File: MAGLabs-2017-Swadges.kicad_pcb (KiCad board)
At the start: 2 copper layers, 70 x 120 mm, 37 parts, among them J1 LCD Screen, J2 IR Sensor, J3 Program, U1 ESP12E

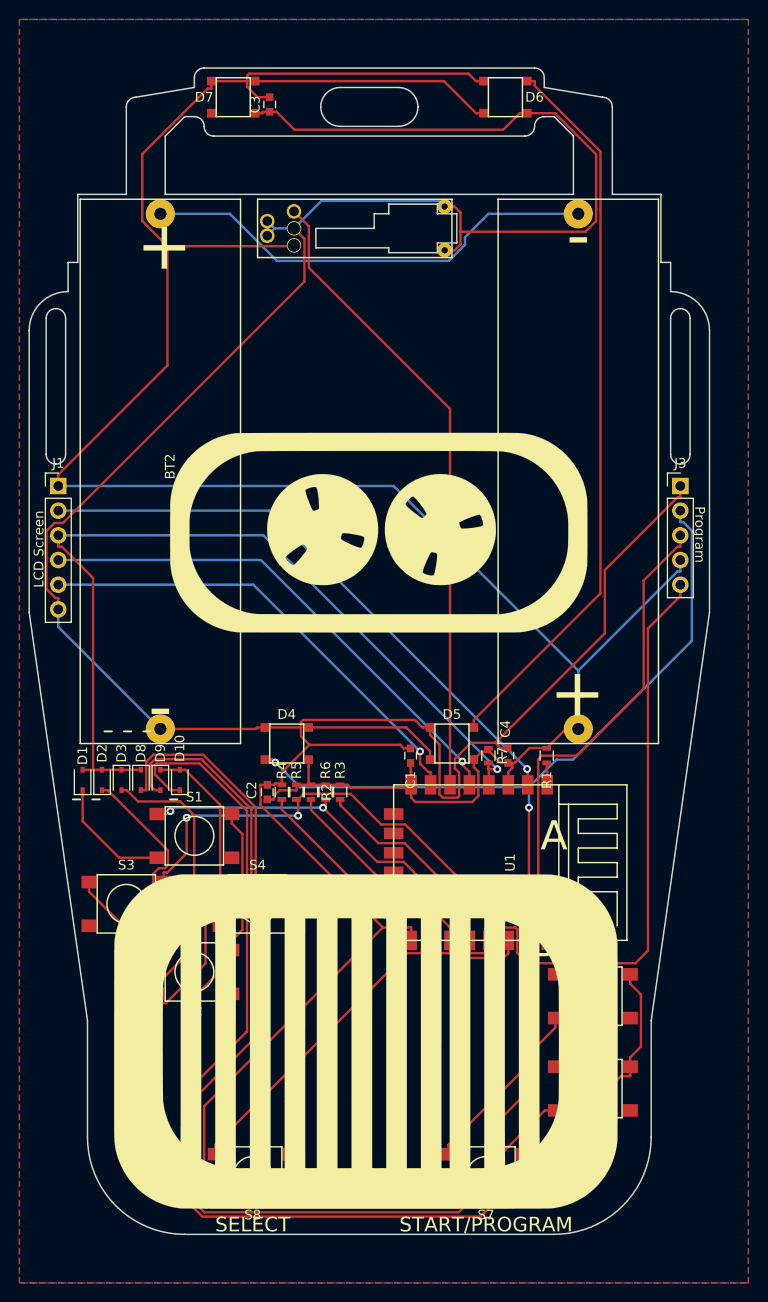
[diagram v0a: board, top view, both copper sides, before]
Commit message: Citizen
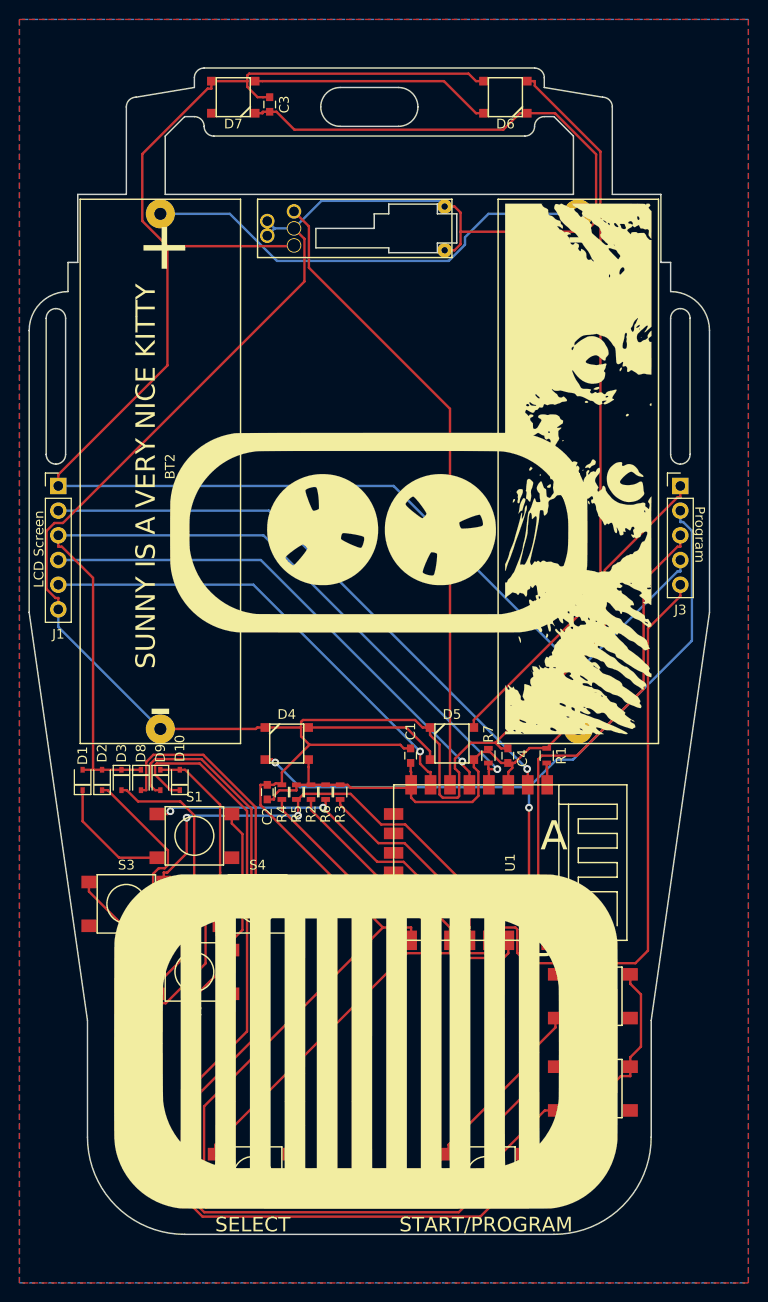
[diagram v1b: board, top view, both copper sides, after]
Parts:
- added G***: LOGO, local:SUNNY, F.Cu at (157.5, 76.2)
- added G***: LOGO, local:Citizen-label, B.Cu at (136.0, 119.0)
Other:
- rule pad_to_mask_clearance: 0.2 -> 0.1
- board text added: "SUNNY IS A VERY NICE KITTY"
